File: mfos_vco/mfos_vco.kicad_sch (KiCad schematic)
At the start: 26 parts, among them Q1 SSM2210, U1 OP275

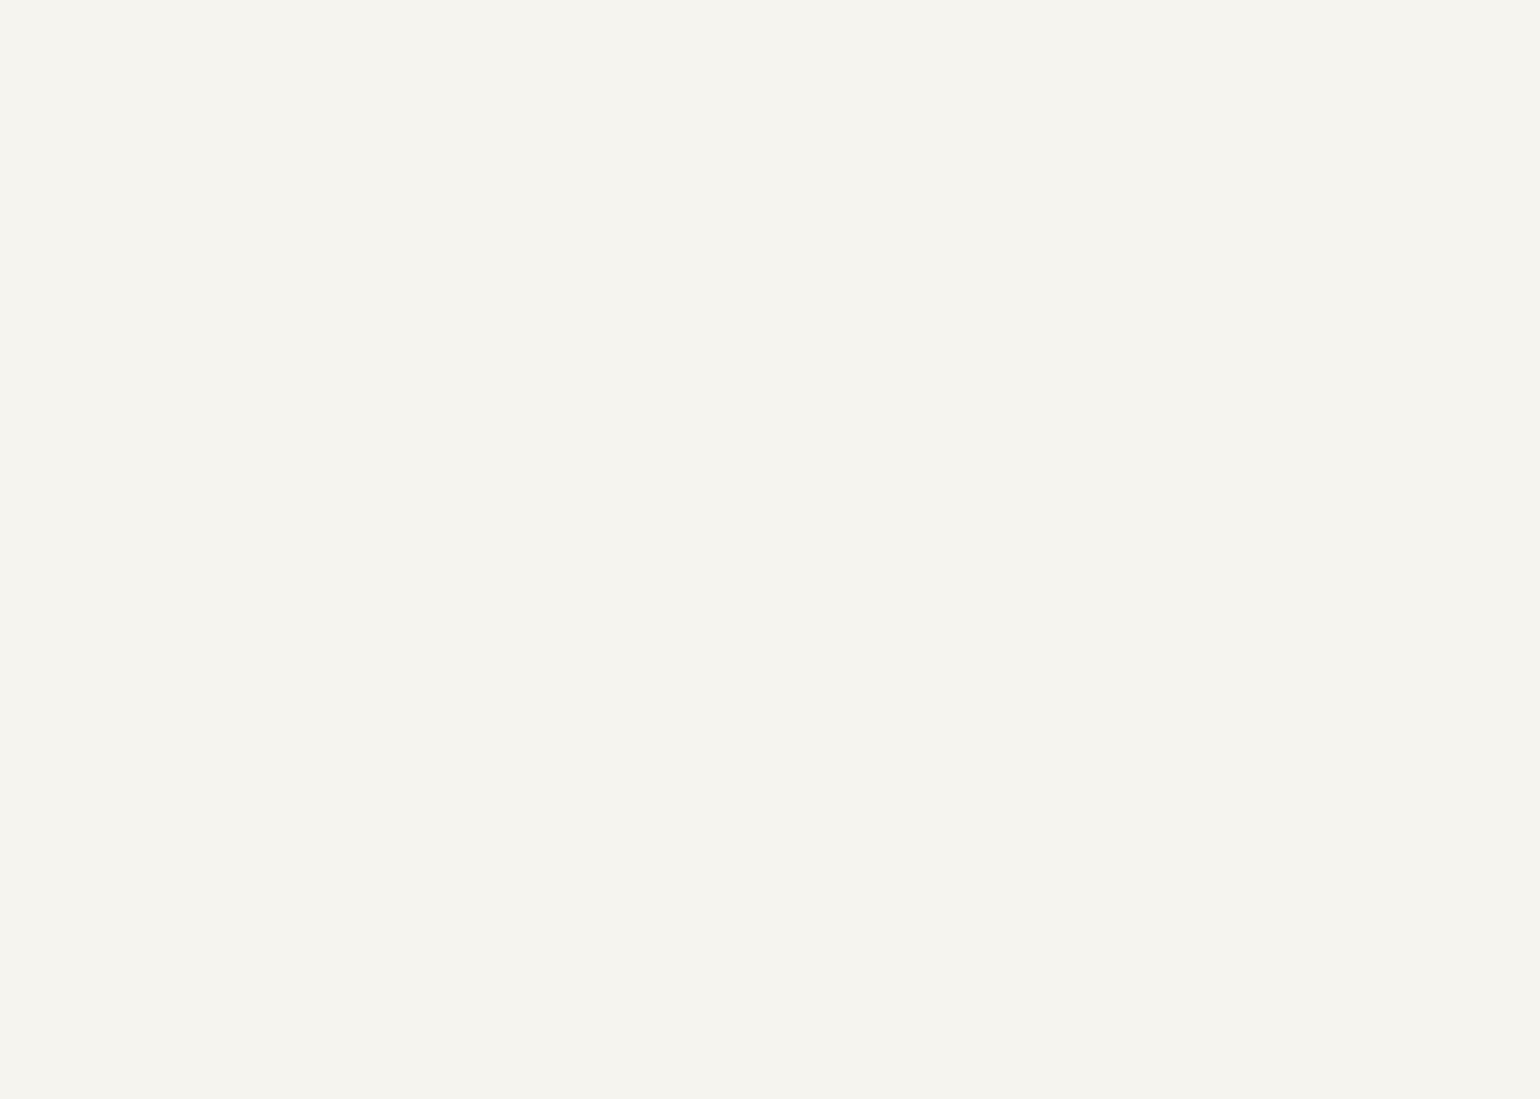
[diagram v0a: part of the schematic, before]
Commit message: Second Commit
nueva hoja
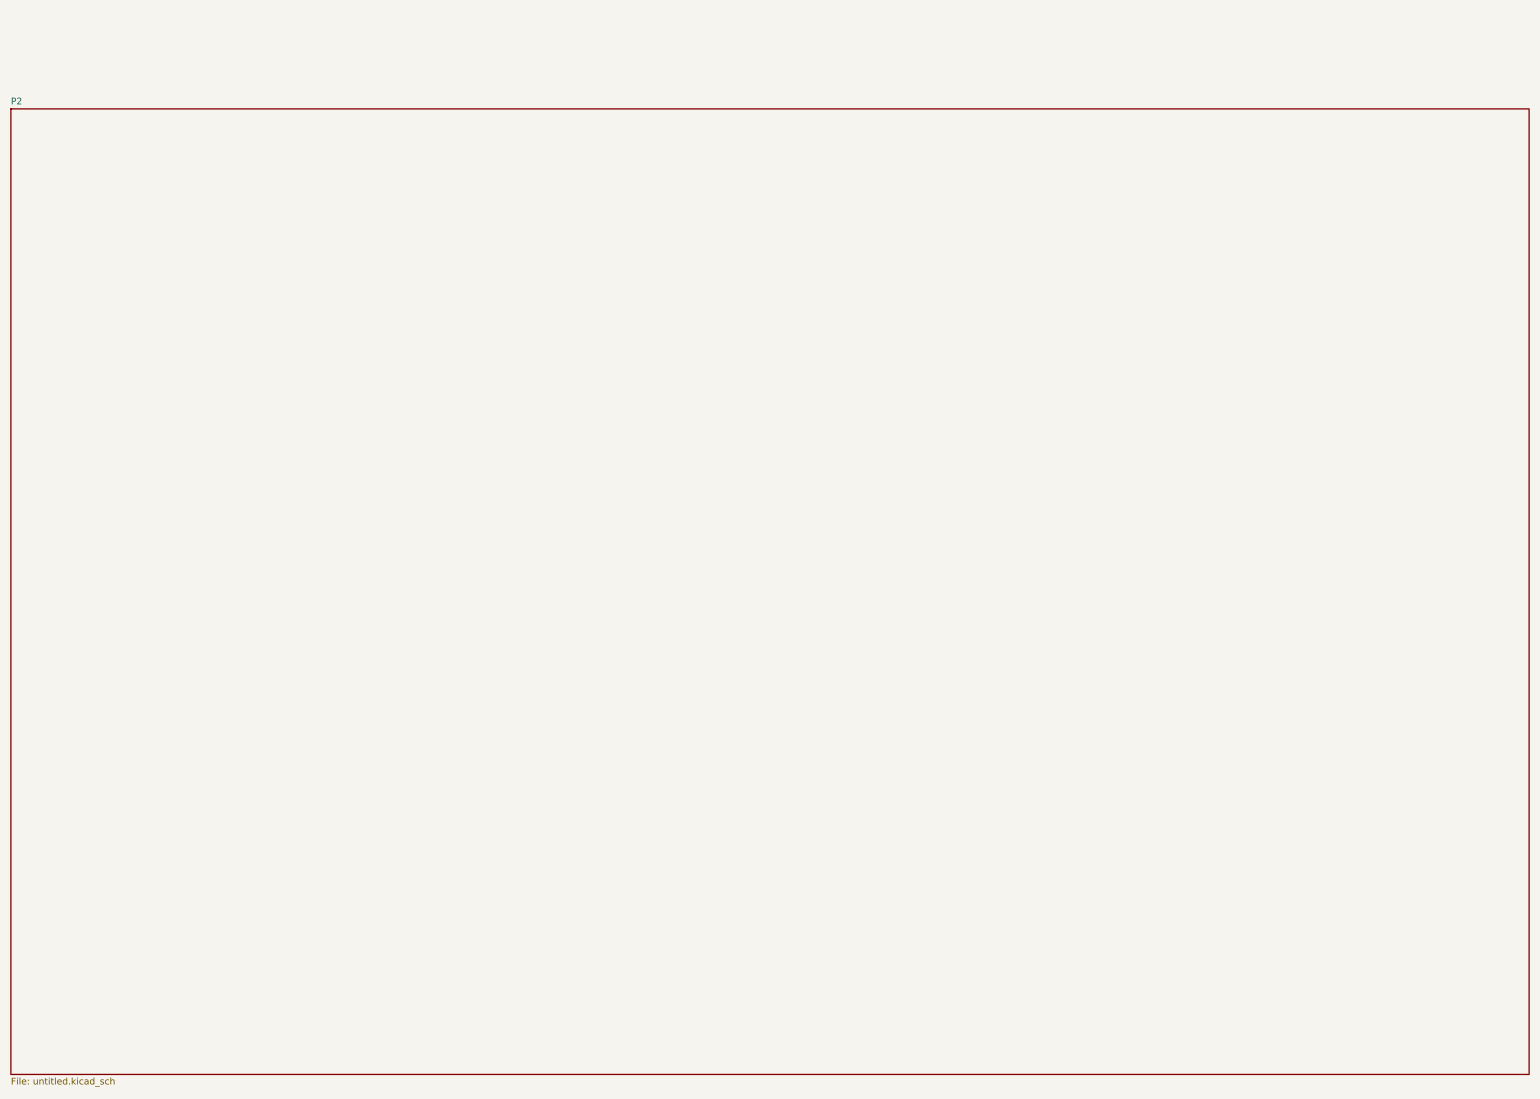
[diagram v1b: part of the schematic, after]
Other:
- added sheet P2 (untitled.kicad_sch)
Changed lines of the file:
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@@
+		)
+	)
+	(sheet
+		(at 5.08 276.86)
+		(size 289.56 184.15)
+		(fields_autoplaced yes)
+		(stroke
+			(width 0.1524)
+			(type solid)
+		)
+		(fill
+			(color 0 0 0 0.0000)
+		)
+		(property "Sheetname" "P2"
+			(at 5.08 276.1484 0)
+			(effects
+				(font
+					(size 1.27 1.27)
+				)
+				(justify left bottom)
+			)
+		)
+		(property "Sheetfile" "untitled.kicad_sch"
+			(at 5.08 461.5946 0)
+			(effects
+				(font
+					(size 1.27 1.27)
+				)
+				(justify left top)
+			)
+		)
+		(instances
+			(project "mfos_vco"
+				(path "/db27d43e-bcf4-48a8-8785-18123cee165a"
+					(page "2")
+				)
+			)
 		)
 	)

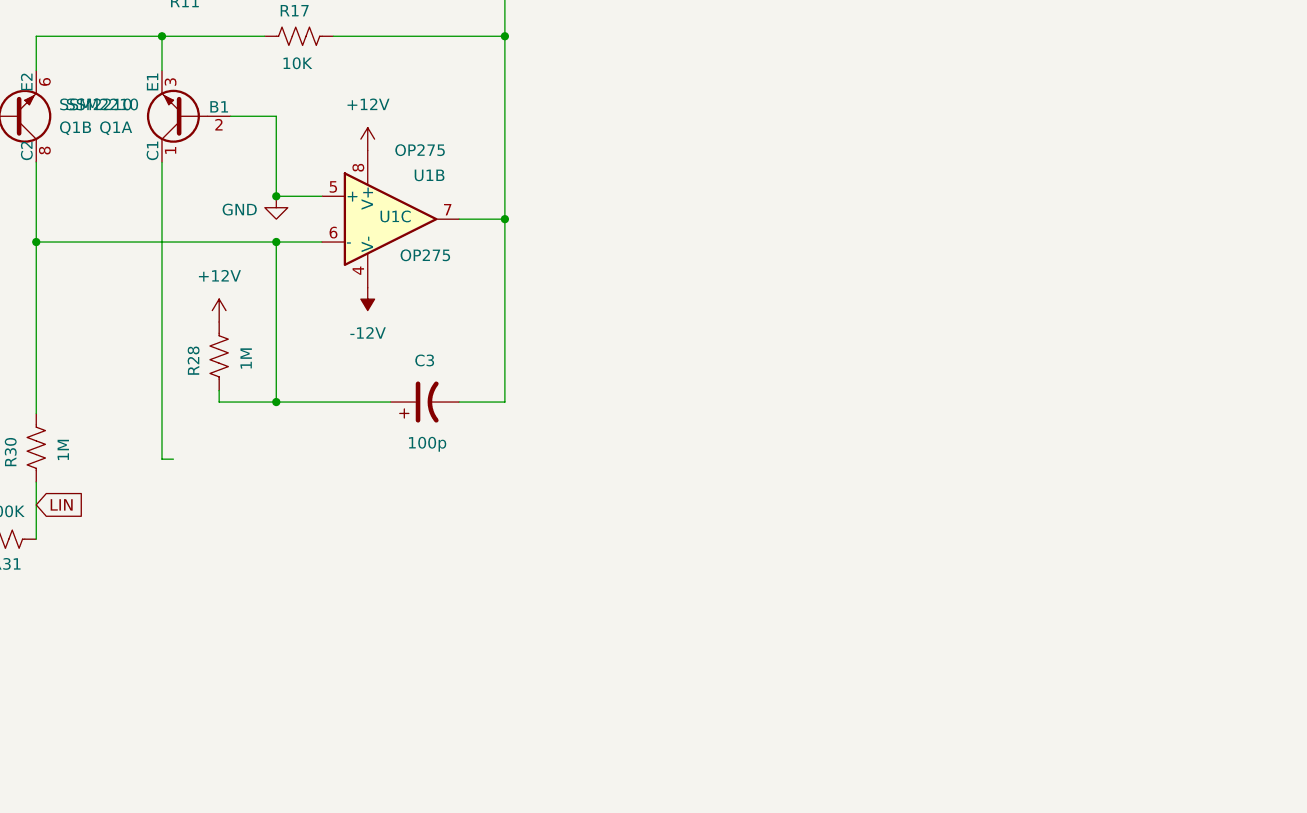
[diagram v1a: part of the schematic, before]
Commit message: update
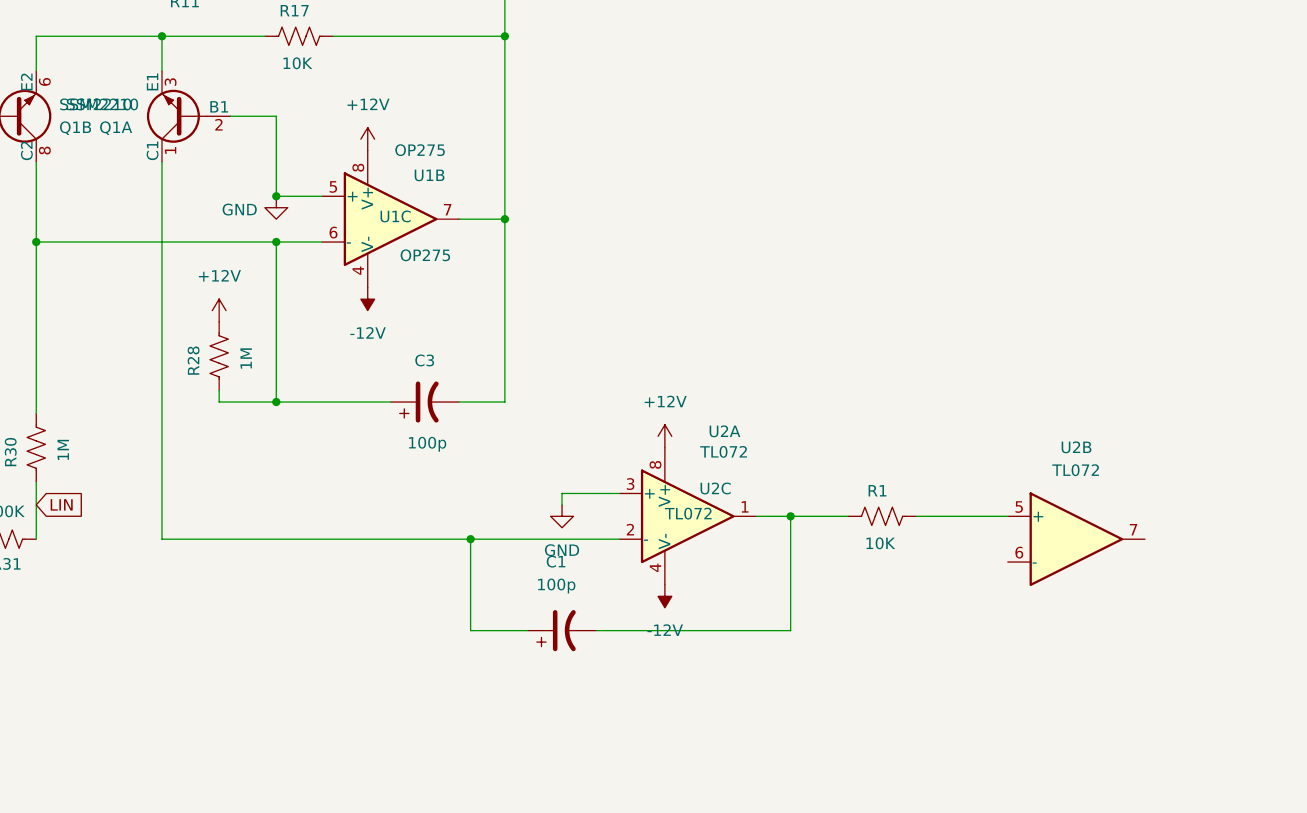
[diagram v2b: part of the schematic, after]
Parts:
- added C1: 100p, symbol Device:C_Polarized_US
- added R1: 10K, symbol Device:R_US
- added U2: TL072, symbol Amplifier_Operational:TL072
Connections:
- net +12V: now also U2.8 (V+)
- net -12V: now also U2.4 (V-)
- net GND: now also U2.3 (+)
- net at Q1.1 (C1): now also C1.1, U2.2 (-)
- new net: R1.1, U2.5 (+)
- new net: C1.2, R1.2, U2.1

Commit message: added gitignore and updated to kicad 9
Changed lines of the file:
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@@
 (kicad_sch
-	(version 20231120)
+	(version 20250114)
 	(generator "eeschema")
-	(generator_version "8.0")
+	(generator_version "9.0")
 	(paper "A4")
+	(text "COARSE\n"
+		(exclude_from_sim no)
+		(at 64.516 63.246 0)
+		(effects
+			(font
+				(size 1.27 1.27)
+			)
+		)
+	)
+	(text "FINE\n"
+		(exclude_from_sim no)
+		(at 74.676 50.546 0)
+		(effects
+			(font
+				(size 1.27 1.27)
+			)
+		)
+	)
 	(junction
 		(at 86.36 123.19)
@@
 		)
 	)
-	(text "COARSE\n"
-		(exclude_from_sim no)
-		(at 64.516 63.246 0)
-		(effects
-			(font
-				(size 1.27 1.27)
-			)
-		)
-	)
-	(text "FINE\n"
-		(exclude_from_sim no)
-		(at 74.676 50.546 0)
-		(effects
-			(font
-				(size 1.27 1.27)
-			)
-		)
-	)
 	(global_label "CV3"
 		(shape input)
@@
 		(at 5.08 276.86)
 		(size 289.56 184.15)
+		(exclude_from_sim no)
+		(in_bom yes)
+		(on_board yes)
+		(dnp no)
 		(fields_autoplaced yes)
 		(stroke
@@
 		)
 	)
+	(embedded_fonts no)
 )
